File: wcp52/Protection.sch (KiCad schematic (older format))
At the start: 14 parts

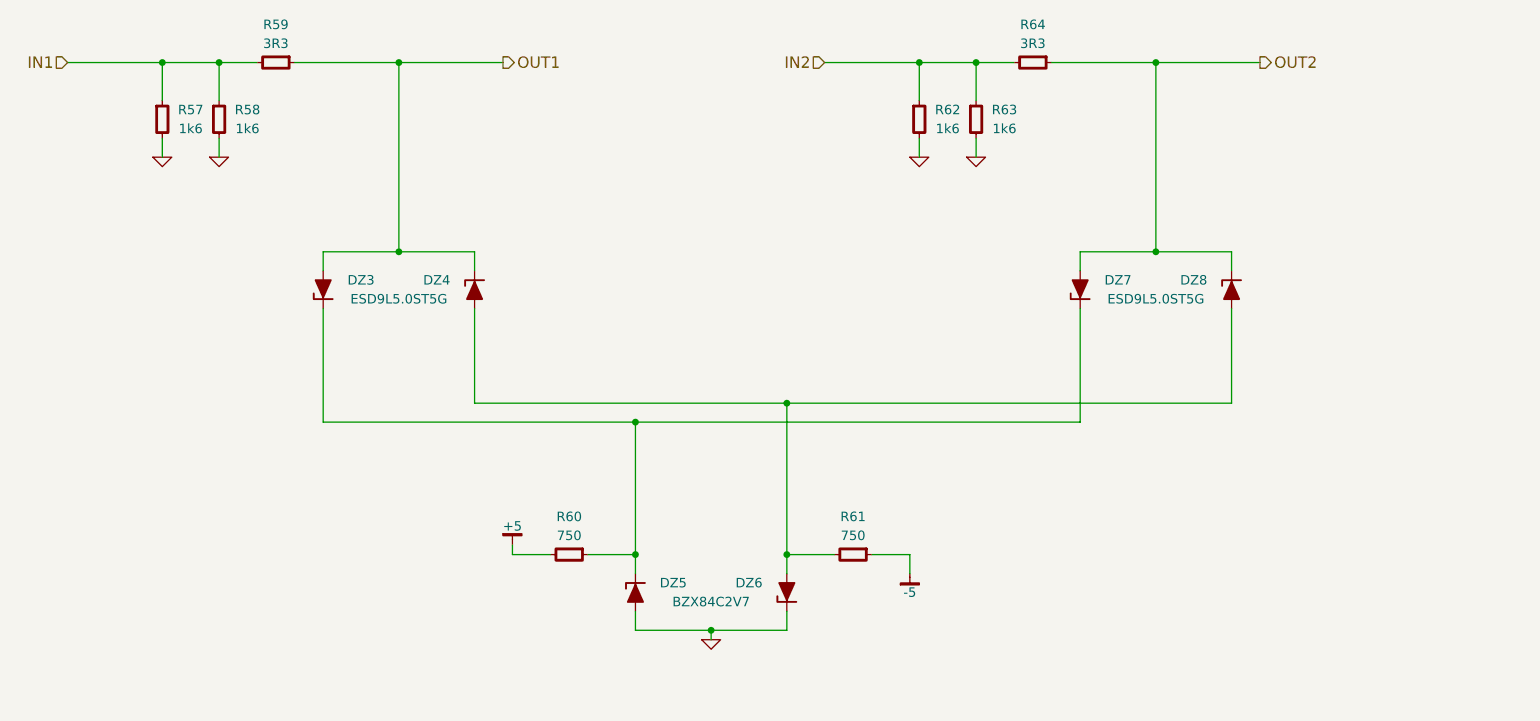
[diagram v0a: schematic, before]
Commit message: Schematic touchups
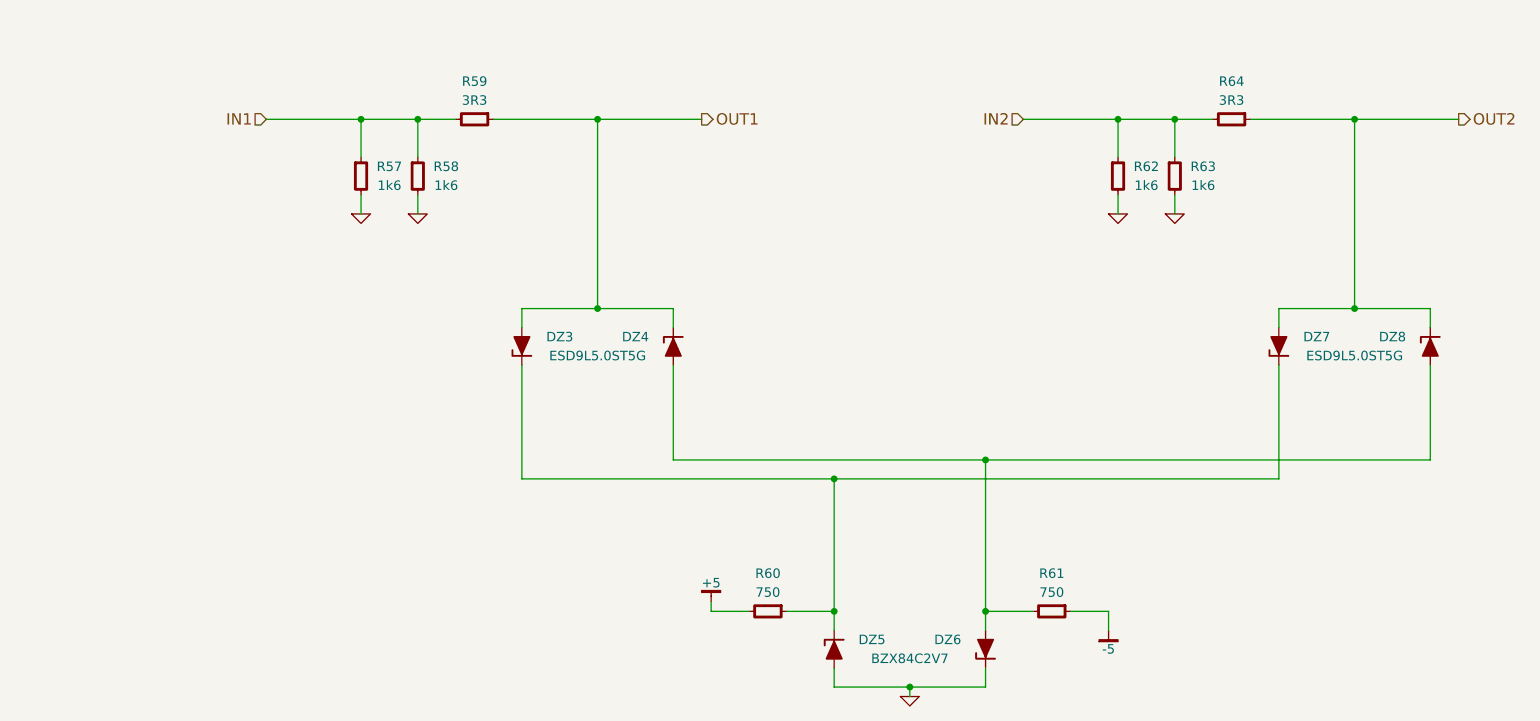
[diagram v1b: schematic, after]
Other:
- moved on the sheet: DZ3, DZ4, DZ5, DZ6, DZ7, DZ8, R57, R58, R59, R60, R61, R62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
